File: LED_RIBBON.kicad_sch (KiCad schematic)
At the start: 21 parts, among them J10 Conn_02x02_Odd_Even, J11 Conn_02x02_Odd_Even, J12 Conn_02x02_Odd_Even, J13 Conn_02x02_Odd_Even, J14 Conn_02x02_Odd_Even, J15 Conn_02x02_Odd_Even, J16 Conn_02x02_Odd_Even, J17 Conn_02x02_Odd_Even, U13 TCA9617A

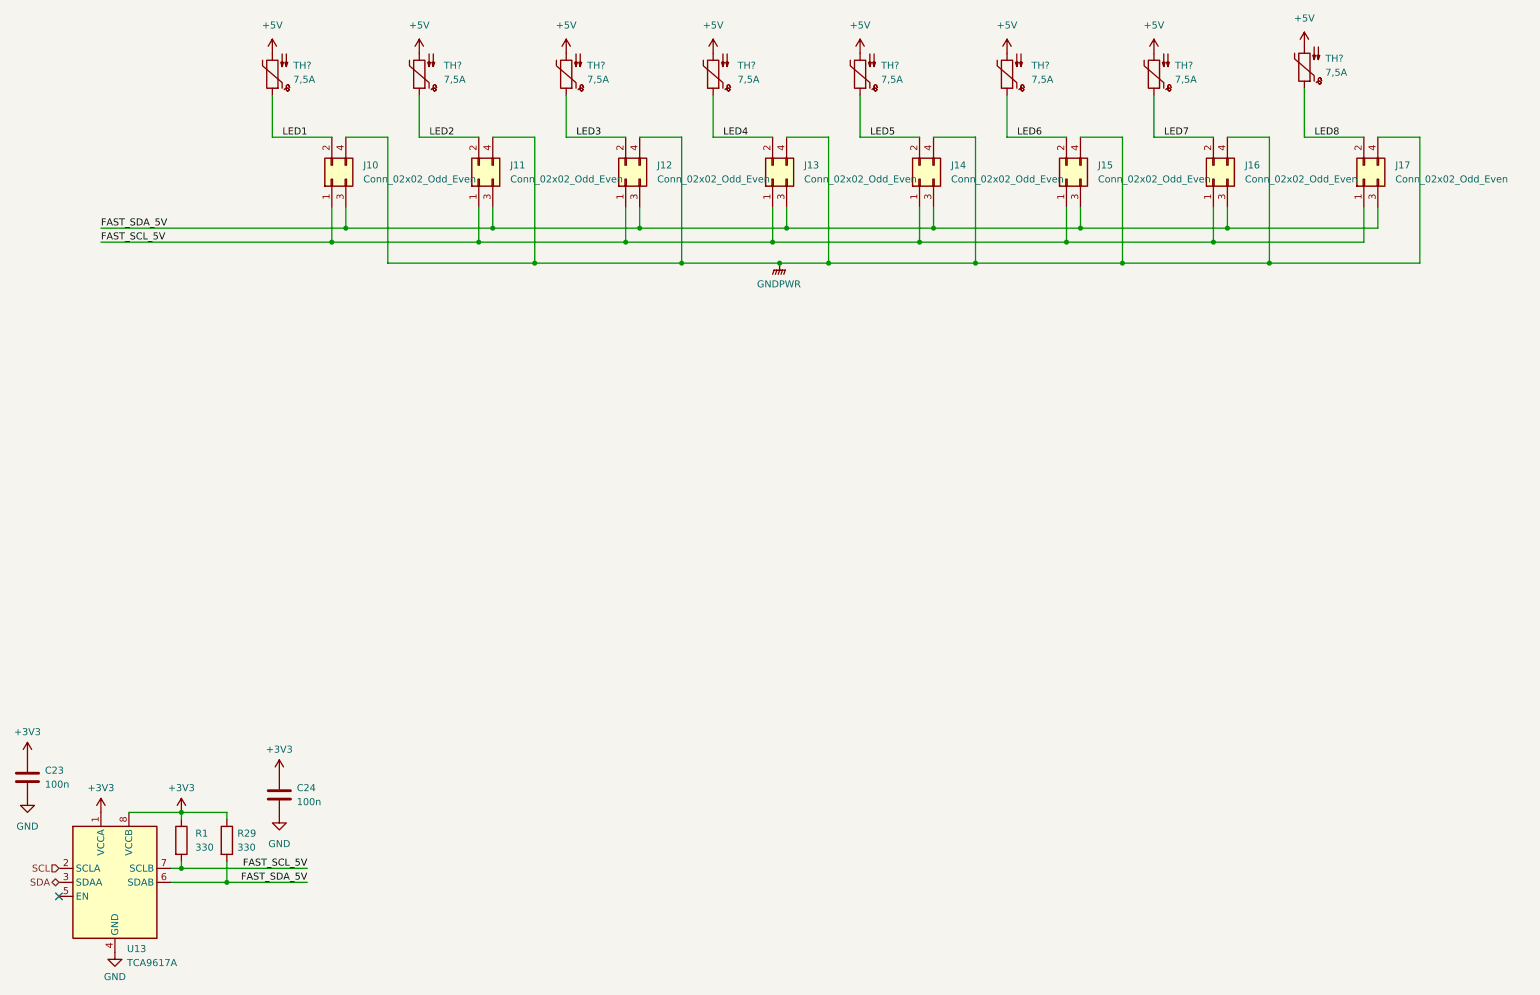
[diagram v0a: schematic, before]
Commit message: JLCJLCJLCJLC
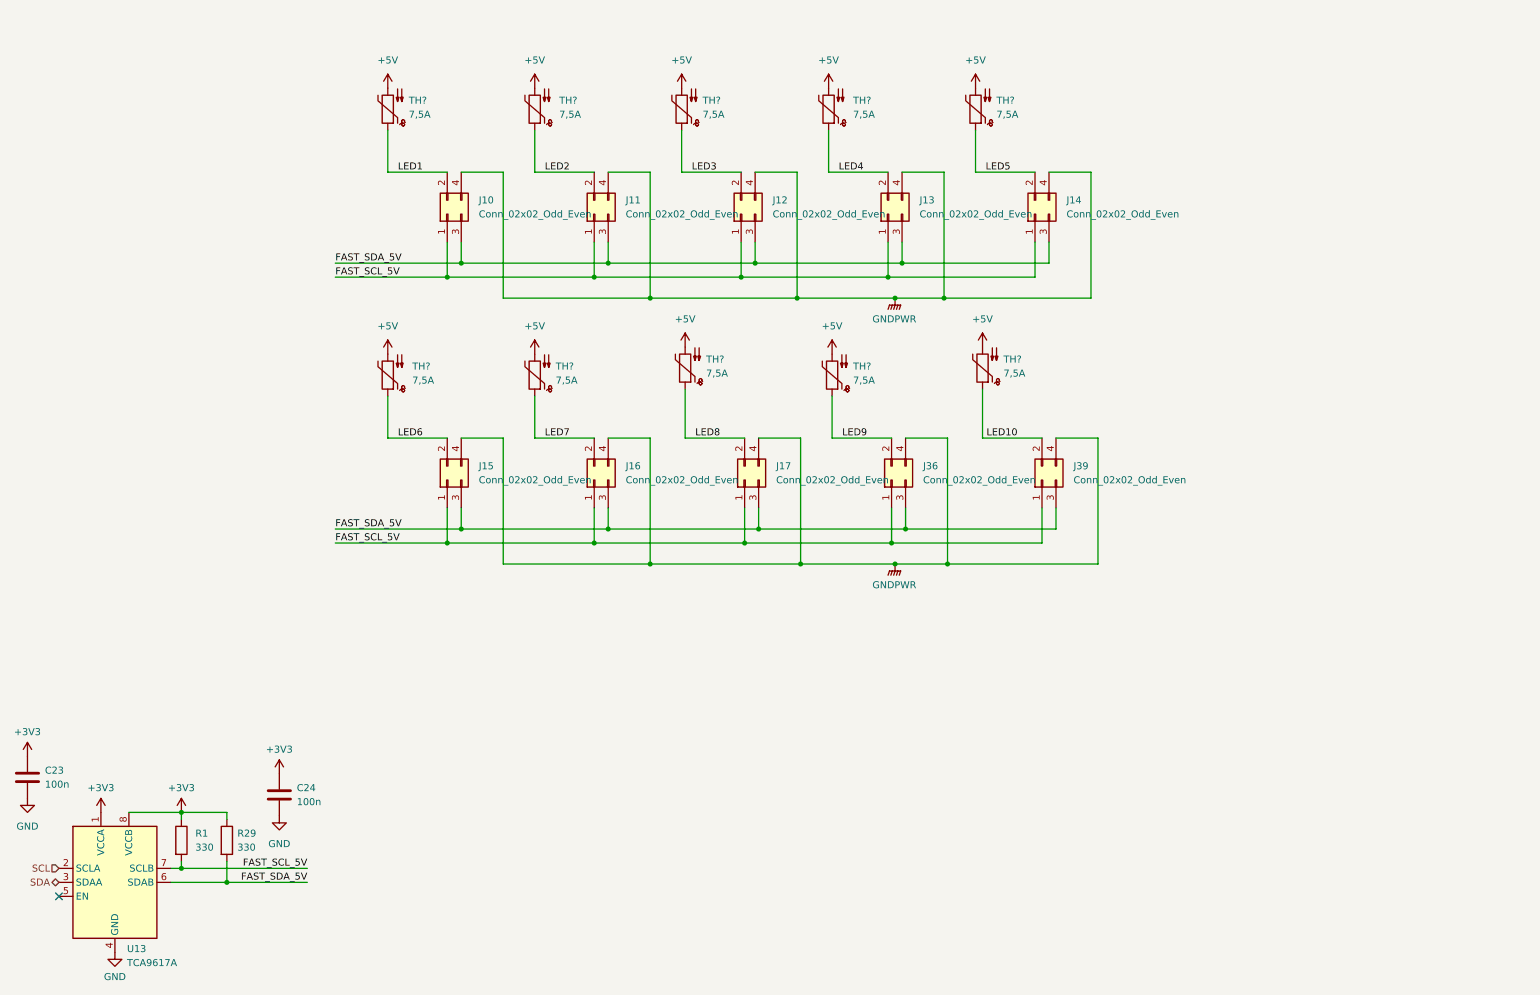
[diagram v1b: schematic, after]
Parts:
- added J36, J39: Conn_02x02_Odd_Even, Connector_Molex:Molex_Mini-Fit_Jr_5566-04A_2x02_P4.20mm_Vertical, symbol Connector_Generic:Conn_02x02_Odd_Even
- added TH? (x2): 7,5A, Resistor_SMD:R_1210_3225Metric, symbol Device:Thermistor_PTC
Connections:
- net +5V: now also TH?.2, TH?.2
- net FAST_SCL_5V: now also J36.1 (Pin_1), J39.1 (Pin_1)
- net FAST_SDA_5V: now also J36.3 (Pin_3), J39.3 (Pin_3)
- net GNDPWR: now also J36.4 (Pin_4), J39.4 (Pin_4)
- new net LED10: J39.2 (Pin_2), TH?.1
- new net LED9: J36.2 (Pin_2), TH?.1
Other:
- moved on the sheet: J10, J11, J12, J13, J14, J15, J16, J17, TH?

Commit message: Before flip
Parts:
- J10, J11, J12, J13, J14, J15, J16, J17, J36, J39: mouser (none) -> 649-10127820-0422PLF; mouser2 (none) -> 571-1586019-4
- R1, R29: mouser (none) -> 603-RT1206FRE07330RL
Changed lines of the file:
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@@
+      (effects (font (size 1.27 1.27)) hide)
+    )
+    (property "mouser" " 649-10127820-0422PLF " (at 96.52 52.07 0)
+      (effects (font (size 1.27 1.27)) hide)
+    )
+    (property "mouser2" " 571-1586019-4 " (at 96.52 52.07 0)
+      (effects (font (size 1.27 1.27)) hide)
+    )
+    (property "tme" "" (at 96.52 52.07 0)
       (effects (font (size 1.27 1.27)) hide)
     )
@@
       (effects (font (size 1.27 1.27)) hide)
     )
+    (property "mouser2" "" (at 85.725 81.28 0)
+      (effects (font (size 1.27 1.27)) hide)
+    )
     (pin "1")
     (pin "2")
@@
       (effects (font (size 1.27 1.27)) hide)
     )
+    (property "mouser2" "" (at 192.405 33.02 0)
+      (effects (font (size 1.27 1.27)) hide)
+    )
     (pin "1")
     (pin "2")
@@
       (effects (font (size 1.27 1.27)) hide)
     )
+    (property "mouser" " 649-10127820-0422PLF " (at 96.52 100.33 0)
+      (effects (font (size 1.27 1.27)) hide)
+    )
+    (property "mouser2" " 571-1586019-4 " (at 96.52 100.33 0)
+      (effects (font (size 1.27 1.27)) hide)
+    )
+    (property "tme" "" (at 96.52 100.33 0)
+      (effects (font (size 1.27 1.27)) hide)
+    )
     (pin "4")
     (pin "1")
@@
       (effects (font (size 1.27 1.27)) hide)
     )
+    (property "mouser2" "" (at 139.7 80.01 0)
+      (effects (font (size 1.27 1.27)) hide)
+    )
     (pin "1")
     (pin "2")
@@
       (effects (font (size 1.27 1.27)) hide)
     )
+    (property "mouser" " 649-10127820-0422PLF " (at 149.86 52.07 0)
+      (effects (font (size 1.27 1.27)) hide)
+    )
+    (property "mouser2" " 571-1586019-4 " (at 149.86 52.07 0)
+      (effects (font (size 1.27 1.27)) hide)
+    )
+    (property "tme" "" (at 149.86 52.07 0)
+      (effects (font (size 1.27 1.27)) hide)
+    )
     (pin "4")
     (pin "1")
@@
       (effects (font (size 1.27 1.27)) hide)
     )
+    (property "mouser2" "" (at 166.37 81.28 0)
+      (effects (font (size 1.27 1.27)) hide)
+    )
     (pin "1")
     (pin "2")
@@
       (effects (font (size 1.27 1.27)) hide)
     )
+    (property "mouser2" "" (at 193.675 80.01 0)
+      (effects (font (size 1.27 1.27)) hide)
+    )
     (pin "1")
     (pin "2")
@@
       (effects (font (size 1.27 1.27)) hide)
     )
+    (property "mouser2" "" (at 139.065 33.02 0)
+      (effects (font (size 1.27 1.27)) hide)
+    )
     (pin "1")
     (pin "2")
@@
       (effects (font (size 1.27 1.27)) hide)
     )
+    (property "mouser" " 649-10127820-0422PLF " (at 177.165 100.33 0)
+      (effects (font (size 1.27 1.27)) hide)
+    )
+    (property "mouser2" " 571-1586019-4 " (at 177.165 100.33 0)
+      (effects (font (size 1.27 1.27)) hide)
+    )
+    (property "tme" "" (at 177.165 100.33 0)
+      (effects (font (size 1.27 1.27)) hide)
+    )
     (pin "4")
     (pin "1")
@@
       (effects (font (size 1.27 1.27)) hide)
     )
+    (property "mouser2" "" (at 85.725 33.02 0)
+      (effects (font (size 1.27 1.27)) hide)
+    )
     (pin "1")
     (pin "2")
@@
       (effects (font (size 1.27 1.27)) hide)
     )
+    (property "mouser2" "" (at 20.32 154.305 0)
+      (effects (font (size 1.27 1.27)) hide)
+    )
     (pin "1")
     (pin "2")
@@
       (effects (font (size 1.27 1.27)) hide)
     )
+    (property "mouser2" "" (at 165.735 33.02 0)
+      (effects (font (size 1.27 1.27)) hide)
+    )
     (pin "1")
     (pin "2")
@@
       (effects (font (size 1.27 1.27)) hide)
     )
+    (property "mouser" " 649-10127820-0422PLF " (at 150.495 100.33 0)
+      (effects (font (size 1.27 1.27)) hide)
+    )
+    (property "mouser2" " 571-1586019-4 " (at 150.495 100.33 0)
+      (effects (font (size 1.27 1.27)) hide)
+    )
+    (property "tme" "" (at 150.495 100.33 0)
+      (effects (font (size 1.27 1.27)) hide)
+    )
     (pin "4")
     (pin "1")
@@
     )
     (property "Datasheet" "~" (at 123.19 100.33 0)
+      (effects (font (size 1.27 1.27)) hide)
+    )
+    (property "mouser" " 649-10127820-0422PLF " (at 123.19 100.33 0)
+      (effects (font (size 1.27 1.27)) hide)
+    )
+    (property "mouser2" " 571-1586019-4 " (at 123.19 100.33 0)
+      (effects (font (size 1.27 1.27)) hide)
+    )
+    (property "tme" "" (at 123.19 100.33 0)
       (effects (font (size 1.27 1.27)) hide)
     )
@@
       (effects (font (size 1.27 1.27)) hide)
     )
+    (property "mouser2" "" (at 112.395 81.28 0)
+      (effects (font (size 1.27 1.27)) hide)
+    )
     (pin "1")
     (pin "2")
@@
       (effects (font (size 1.27 1.27)) hide)
     )
+    (property "mouser" " 649-10127820-0422PLF " (at 176.53 52.07 0)
+      (effects (font (size 1.27 1.27)) hide)
+    )
+    (property "mouser2" " 571-1586019-4 " (at 176.53 52.07 0)
+      (effects (font (size 1.27 1.27)) hide)
+    )
+    (property "tme" "" (at 176.53 52.07 0)
+      (effects (font (size 1.27 1.27)) hide)
+    )
     (pin "4")
     (pin "1")
@@
     )
     (property "Datasheet" "~" (at 123.19 52.07 0)
+      (effects (font (size 1.27 1.27)) hide)
+    )
+    (property "mouser" " 649-10127820-0422PLF " (at 123.19 52.07 0)
+      (effects (font (size 1.27 1.27)) hide)
+    )
+    (property "mouser2" " 571-1586019-4 " (at 123.19 52.07 0)
+      (effects (font (size 1.27 1.27)) hide)
+    )
+    (property "tme" "" (at 123.19 52.07 0)
       (effects (font (size 1.27 1.27)) hide)
     )
@@
       (effects (font (size 1.27 1.27)) hide)
     )
+    (property "mouser2" "" (at 66.04 157.48 0)
+      (effects (font (size 1.27 1.27)) hide)
+    )
     (pin "1")
     (pin "2")
@@
     )
     (property "mouser" " 595-TCA9617ADGKR " (at 36.195 173.355 0)
+      (effects (font (size 1.27 1.27)) hide)
+    )
+    (property "mouser2" "" (at 36.195 173.355 0)
       (effects (font (size 1.27 1.27)) hide)
     )
@@
       (effects (font (size 1.27 1.27)) hide)
     )
+    (property "mouser2" "" (at 48.26 165.735 0)
+      (effects (font (size 1.27 1.27)) hide)
+    )
+    (property "mouser" " 603-RT1206FRE07330RL " (at 48.26 165.735 0)
+      (effects (font (size 1.27 1.27)) hide)
+    )
     (pin "2")
     (pin "1")
@@
       (effects (font (size 1.27 1.27)) hide)
     )
+    (property "mouser" " 649-10127820-0422PLF " (at 204.47 100.33 0)
+      (effects (font (size 1.27 1.27)) hide)
+    )
+    (property "mouser2" " 571-1586019-4 " (at 204.47 100.33 0)
+      (effects (font (size 1.27 1.27)) hide)
+    )
+    (property "tme" "" (at 204.47 100.33 0)
+      (effects (font (size 1.27 1.27)) hide)
+    )
     (pin "4")
     (pin "1")
@@
       (effects (font (size 1.27 1.27)) hide)
     )
+    (property "mouser2" "" (at 112.395 33.02 0)
+      (effects (font (size 1.27 1.27)) hide)
+    )
     (pin "1")
     (pin "2")
@@
       (effects (font (size 1.27 1.27)) hide)
     )
+    (property "mouser" " 649-10127820-0422PLF " (at 203.2 52.07 0)
+      (effects (font (size 1.27 1.27)) hide)
+    )
+    (property "mouser2" " 571-1586019-4 " (at 203.2 52.07 0)
+      (effects (font (size 1.27 1.27)) hide)
+    )
+    (property "tme" "" (at 203.2 52.07 0)
+      (effects (font (size 1.27 1.27)) hide)
+    )
     (pin "4")
     (pin "1")
@@
       (effects (font (size 1.27 1.27)) hide)
     )
+    (property "mouser2" "" (at 56.515 165.735 0)
+      (effects (font (size 1.27 1.27)) hide)
+    )
+    (property "mouser" " 603-RT1206FRE07330RL " (at 56.515 165.735 0)
+      (effects (font (size 1.27 1.27)) hide)
+    )
